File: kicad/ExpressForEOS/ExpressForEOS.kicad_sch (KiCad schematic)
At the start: 17 parts, among them J1 Conn_02x17_Counter_Clockwise, U1 74HC4051, U10 74LS08, U11 74LS156, U12 74LS156, U13 74LS373, U14 ICM7218BIPI, U15 MAX150BCPP, U16 LM358, U2 74HC4051, U3 74HC4051, U4 74HC4051, U5 CD4066BE, U6 74LS138, U7 74LS374, U8 74LS374, U9 74LS245

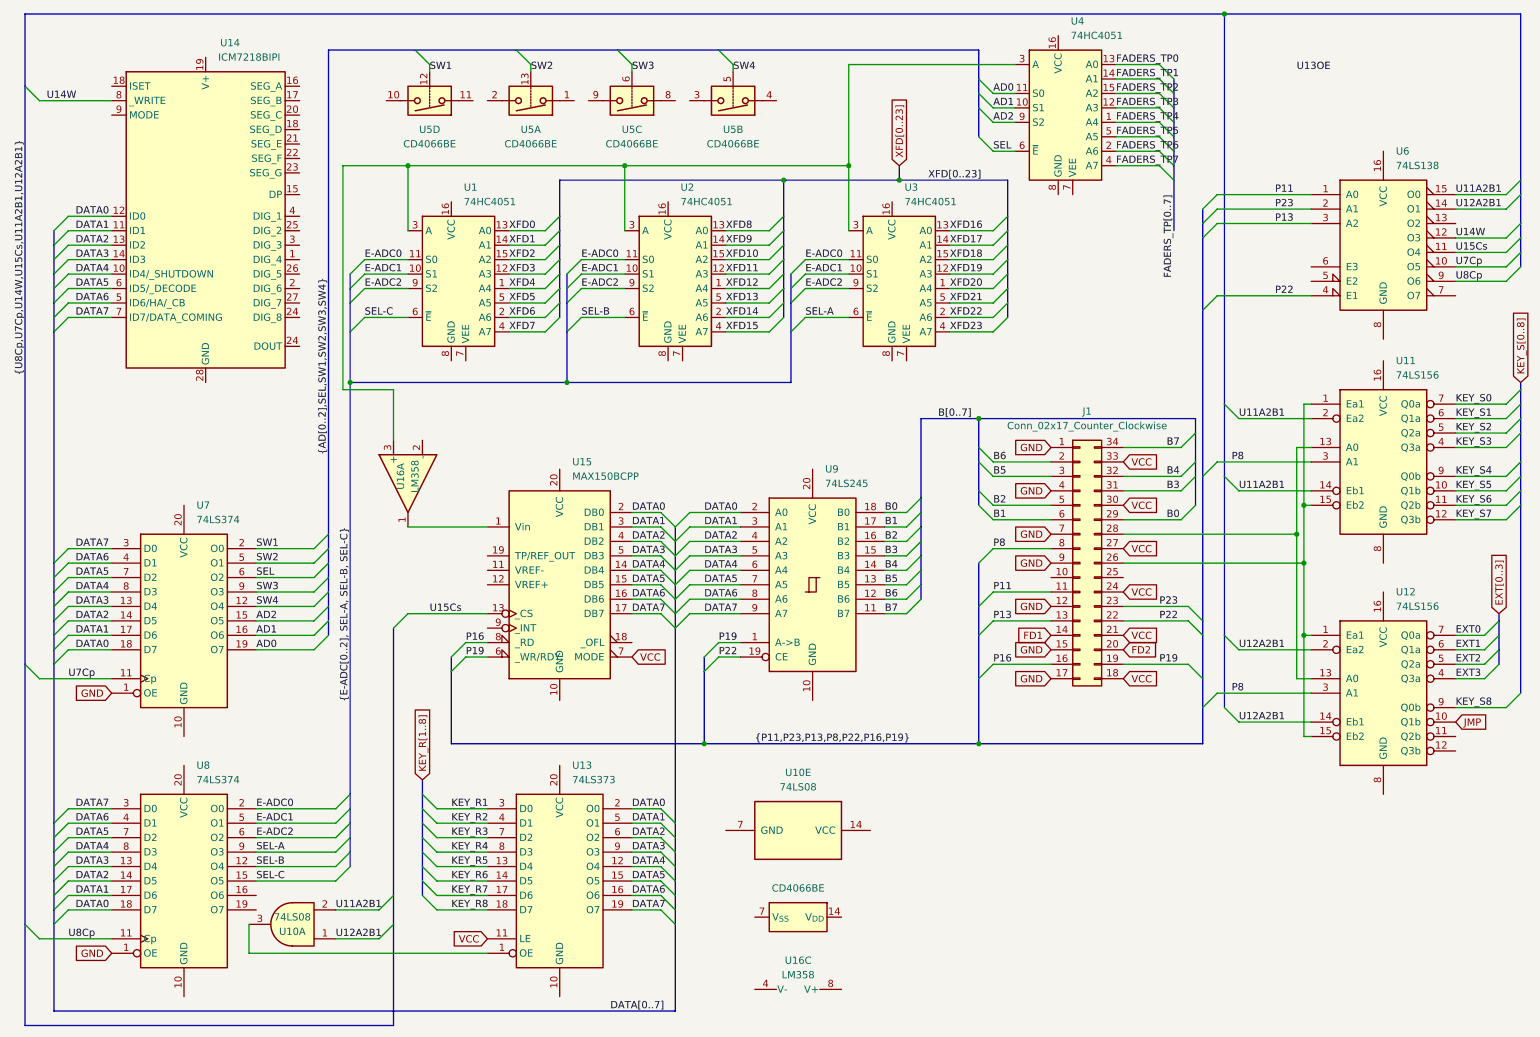
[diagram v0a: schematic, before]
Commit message: Schem update
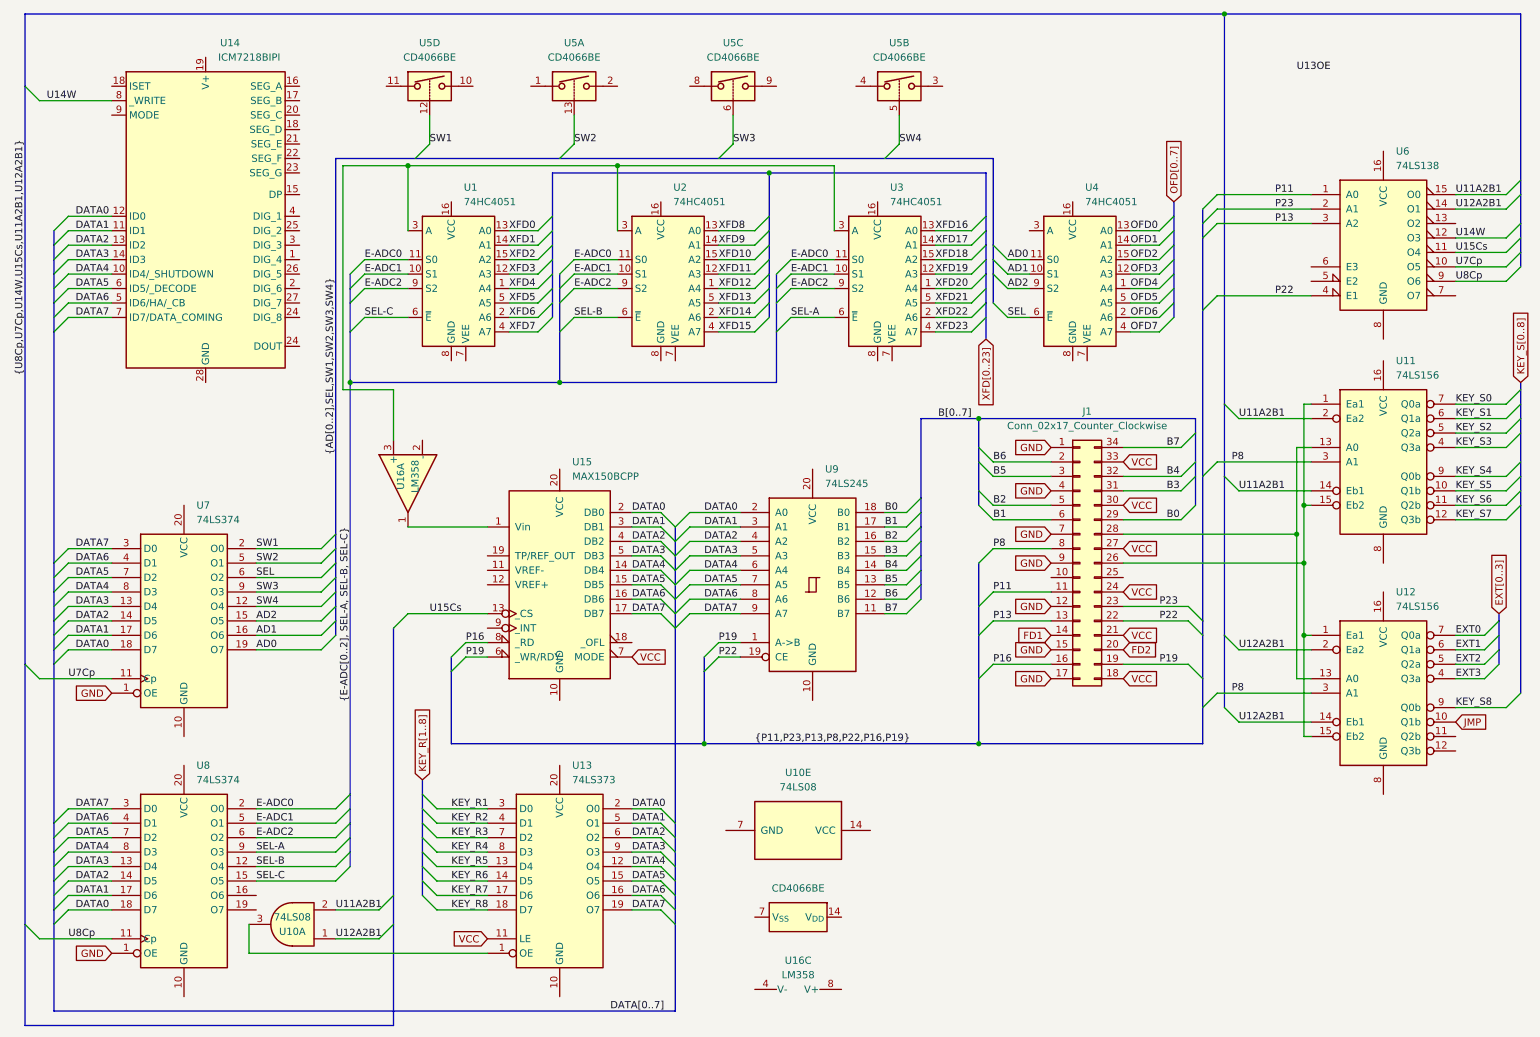
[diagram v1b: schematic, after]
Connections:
- net at U1.3 (A), U16.3 (+), U2.3 (A)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: no longer U4.3 (A)
- net FADERS_TP0 renamed OFD0
- net FADERS_TP1 renamed OFD1
- net FADERS_TP2 renamed OFD2
- net FADERS_TP3 renamed OFD3
- net FADERS_TP4 renamed OFD4
- net FADERS_TP5 renamed OFD5
- net FADERS_TP6 renamed OFD6
- net FADERS_TP7 renamed OFD7
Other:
- moved on the sheet: U2, U3, U4, U5A, U5B, U5C, U5D
